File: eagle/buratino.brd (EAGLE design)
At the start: 25.9 x 61 mm, 51 parts, among them IC1 LTC3105MS, J4 Ext Battery, Q2 2n7002PW, U2 TPS78222, U4 ATMEGA256RFR2, U7 SWITCH, U8 LED-RGB, X1 16MHz, X2 32.768k, X3 AVR_JTAG, Y1 ANTENNA2SMD5

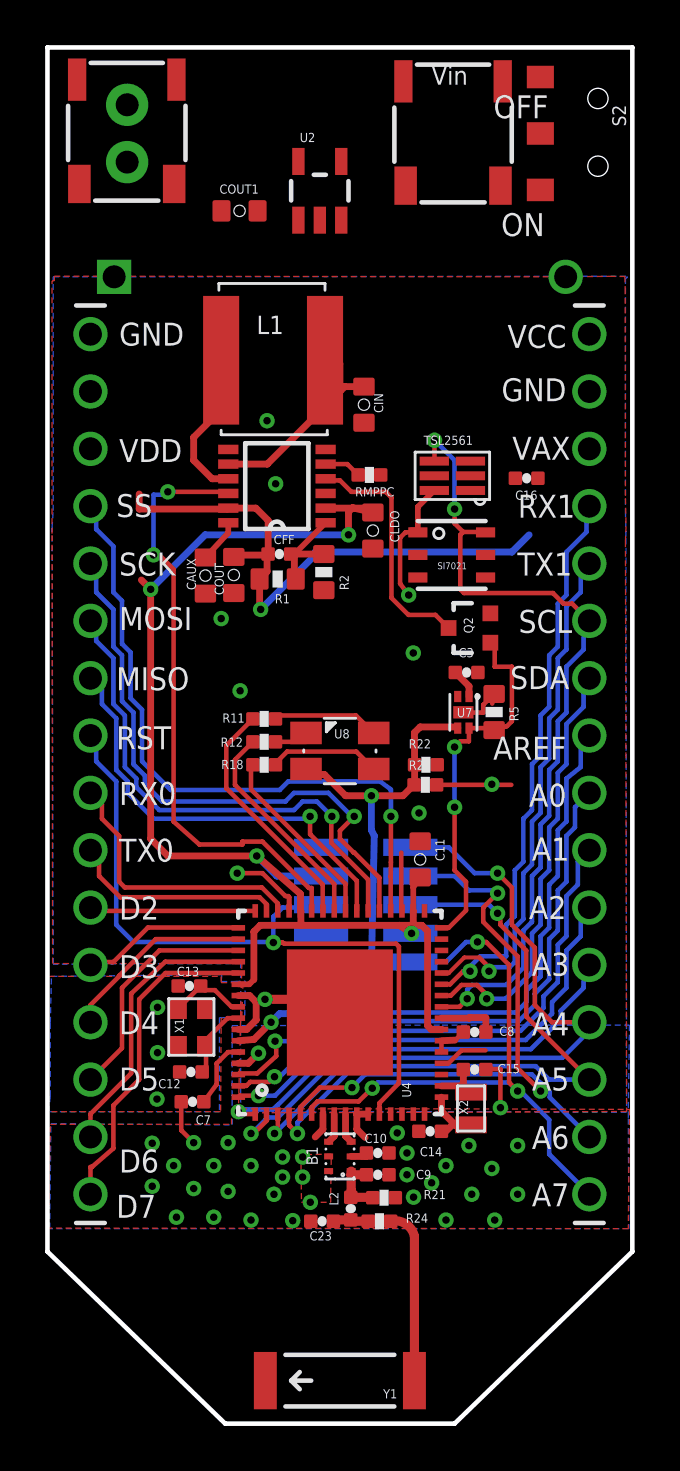
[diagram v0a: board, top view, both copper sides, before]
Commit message: add PIR
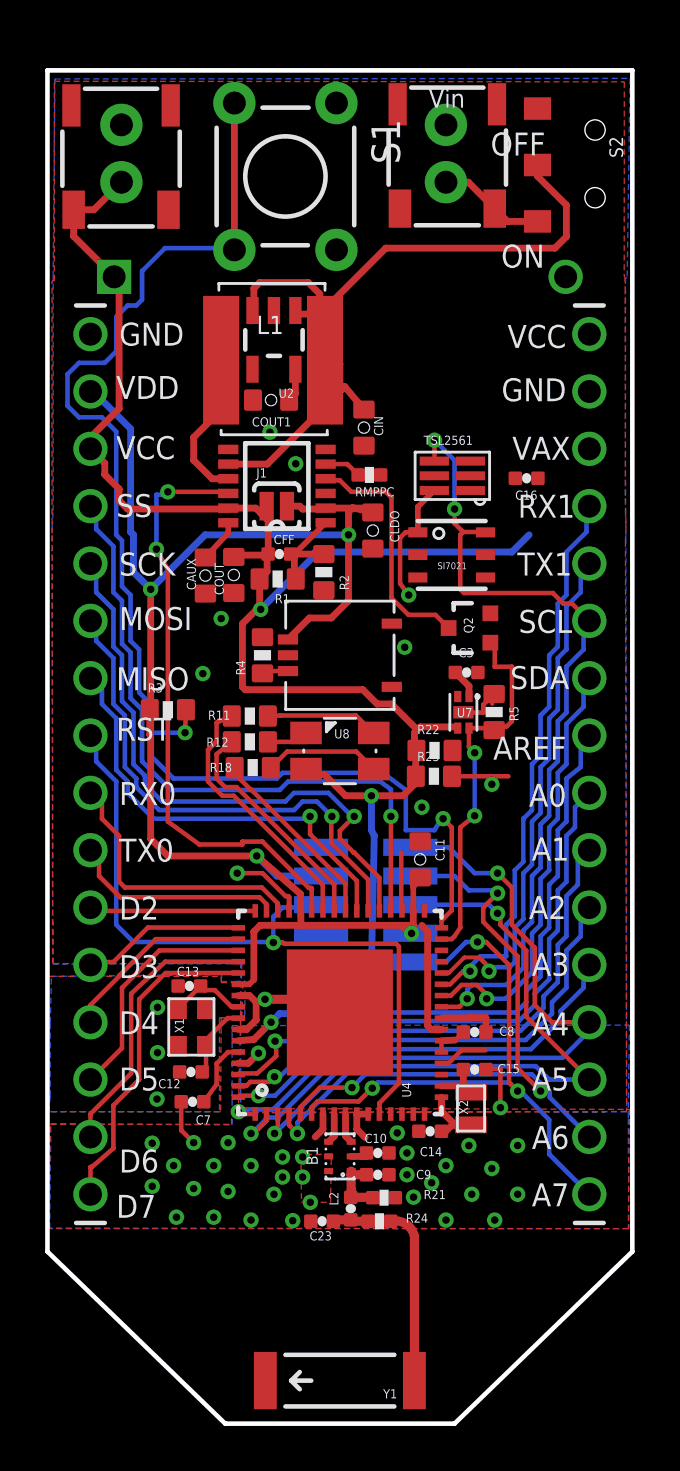
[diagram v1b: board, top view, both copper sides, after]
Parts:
- removed PV: SolarCell, bean:JST-SFH
- added J1: Vcc-Vdd Tie, Pinoccio:SJ_2S-NO
- added J2: Ext Battery, Pinoccio:1X02
- added R3: 10K, Pinoccio:0603-RES
- added R4: 47K, Pinoccio:0603-RES
- added S1: (no value), SparkFun-Electromechanical:TACTILE-PTH
- added U$1: IRS-B210ST01R1, 620-Sensors:PIRSMT
- added VIN1: Ext Power, bean:JST-SFH
- BATT: value JST Bat -> Aux Bat
- J4: value Ext Battery -> Aux Batt
- R11, R12, R18, R22, R23: device Pinoccio:0402-RES -> Pinoccio:0603-RES
- moved COUT1 8.50 mm to (9.65, 45.3), turned to 180 degrees
- moved U2 6.91 mm to (9.78, 48.0), turned to 180 degrees
- moved S2 1.40 mm to (24.0, 55.8)
- moved BATT 1.17 mm to (0.41, 59.1)
- moved CIN 1.02 mm to (13.8, 44.1)
- moved J4 0.92 mm to (3.02, 57.5)
- moved R22 0.74 mm to (16.9, 29.8)
- moved R11 0.65 mm to (8.71, 31.3)
- moved R12 0.64 mm to (8.71, 30.2)
- moved R23 0.54 mm to (16.9, 28.7)
- moved R18 0.52 mm to (8.84, 29.1)
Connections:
- removed net 123: JP-L.2
- removed net N$66: U2.1, U2.3
- removed net N$9: CIN.1, IC1.8, L1.P$1, S2.2
- new net BTN: R3.2, S1.3, S1.4, U4.32
- new net VIN: CIN.1, IC1.8, L1.P$1, S2.2, U2.1, U2.3
- net A0: now also R4.1, U$1.VOUT
- net GND: now also J2.1, R4.2, S1.1, S1.2, U$1.GND, U$1.GND*1, U$1.GND*2, VIN1.2; no longer PV.2
- net N$24: now also J2.2, VIN1.1; no longer PV.1
- net SHDWN: now also U4.31; no longer U4.29, U4.32
- net VCC: now also J1.1, JP-L.3
- net VDD: now also J1.2, JP-L.2, R3.1, U$1.VIN; no longer JP-L.3
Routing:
- net BTN: track 0.00 -> 60.6 mm, vias 0 -> 2
- net VIN: track 0.00 -> 34.9 mm
- net VCC: track 50.5 -> 83.3 mm
- net VDD: track 58.6 -> 76.8 mm
- net N$9: track 9.97 -> 0.00 mm
- net N$24: track 0.00 -> 4.77 mm
- net A0: track 25.0 -> 26.2 mm
- net LED-GRN: track 10.8 -> 11.6 mm
- net SDA: track 28.5 -> 27.7 mm
- net N$1: track 1.75 -> 2.46 mm
- net LED-RED: track 9.65 -> 10.3 mm
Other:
- board size 25.9 x 61 mm -> 25.9 x 59.9 mm
